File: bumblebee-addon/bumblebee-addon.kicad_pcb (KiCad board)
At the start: 2 copper layers, 19 parts, among them J1 RJ25, J2 HEADER, J3 HEADER, J4 ICSP, J5 FTDI_FLASH, J6 INTERFACE, SW1 SW_DIP_x04, U1 ATmega328P-AU, U2 MCP4902, U3 MCP4902

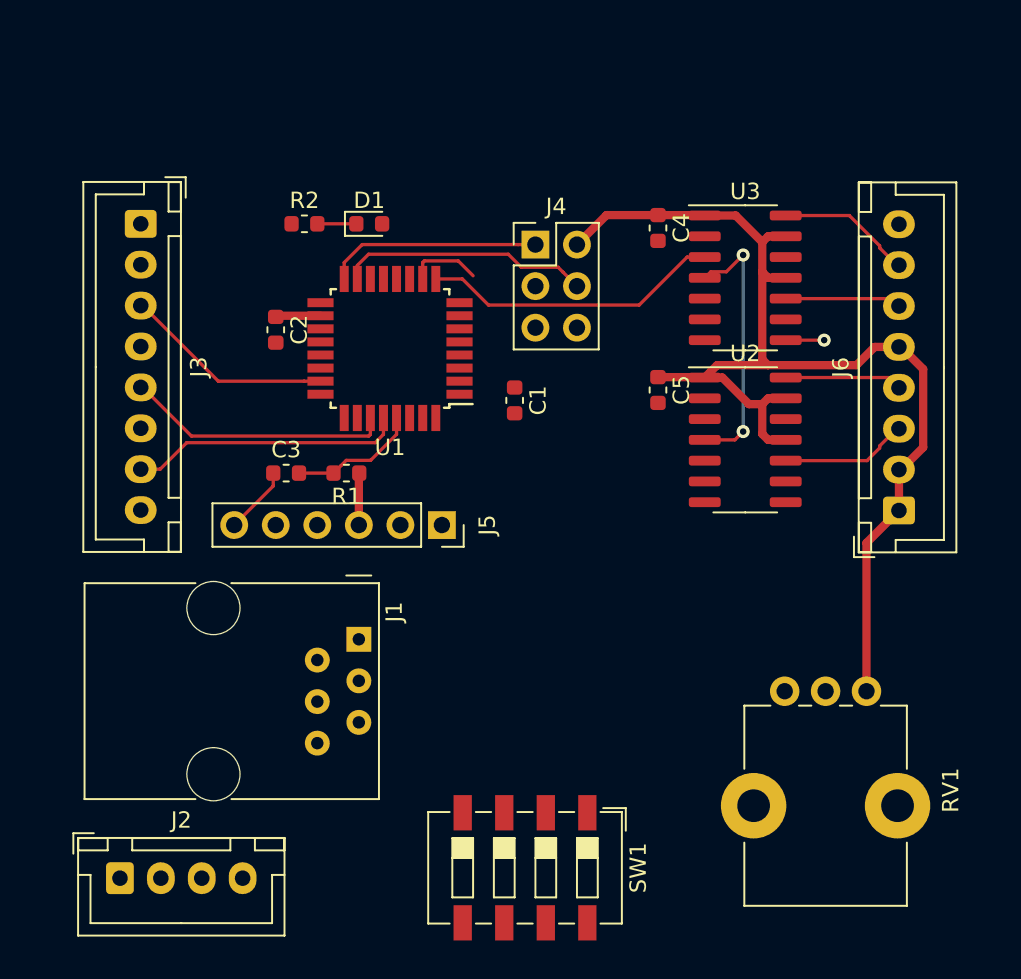
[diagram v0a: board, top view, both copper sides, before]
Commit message: Shipped new revs of all boards.
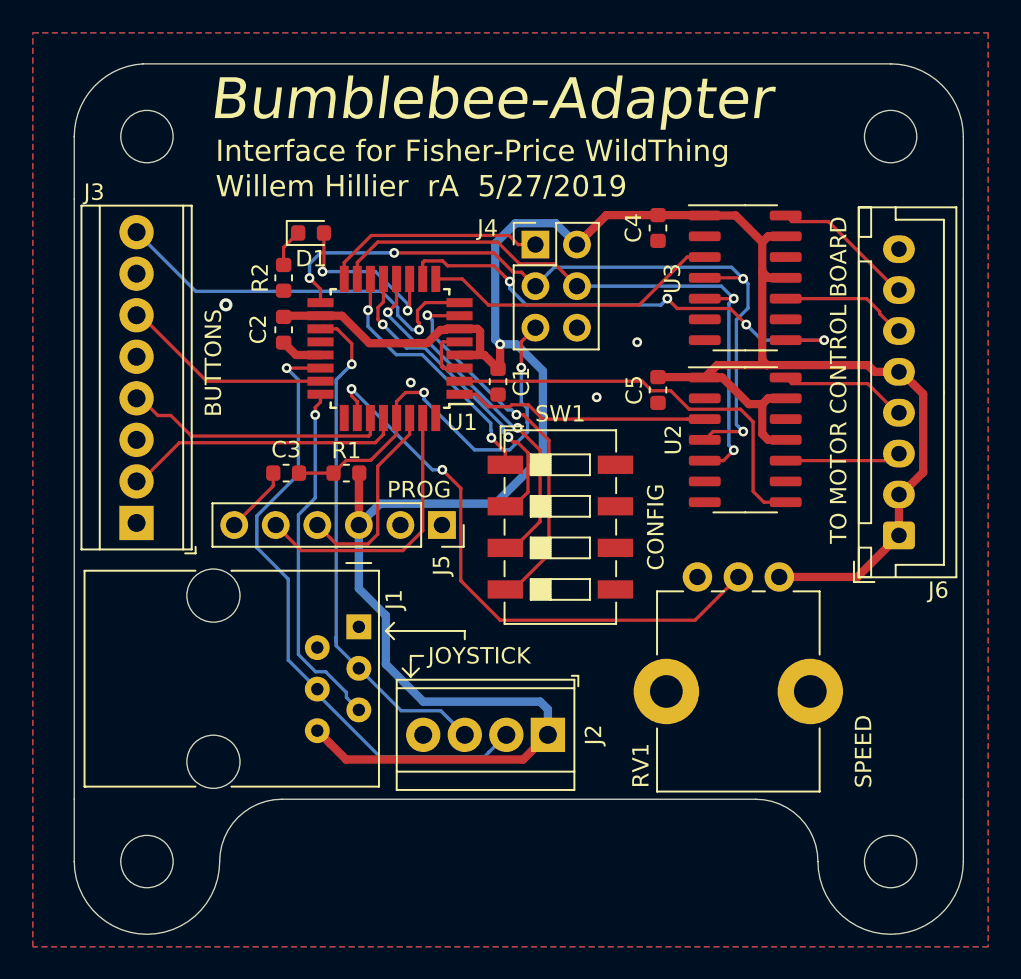
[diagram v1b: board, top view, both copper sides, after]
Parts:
- added G***: LOGO, logo:bumblebee_logo, B.Cu at (149.1, 34.8)
- added REF**: MountingHole_3.2mm_M3, MountingHole:MountingHole_3.2mm_M3, B.Cu at (127.4, 66.9)
- added REF**: MountingHole_3.2mm_M3, MountingHole:MountingHole_3.2mm_M3, F.Cu at (172.8, 66.9)
- added REF**: MountingHole_3.2mm_M3, MountingHole:MountingHole_3.2mm_M3, B.Cu at (172.8, 22.6)
- added REF**: MountingHole_3.2mm_M3, MountingHole:MountingHole_3.2mm_M3, F.Cu at (127.4, 22.6)
- J1: footprint Connector_RJ:RJ12_Amphenol_54601 -> footprints:RJ12_Amphenol_54601
- J2: footprint Connector_JST:JST_XH_B4B-XH-A_1x04_P2.50mm_Vertical -> footprints:TerminalBlock_TE_282834-4_1x04_P2.54mm_Horizontal
- J3: footprint Connector_JST:JST_XH_B8B-XH-A_1x08_P2.50mm_Vertical -> footprints:TerminalBlock_TE_282834-8_1x08_P2.54mm_Horizontal
- RV1: footprint Potentiometer_THT:Potentiometer_Bourns_PTV09A-1_Single_Vertical -> footprints:Potentiometer_Bourns_PTV09A-1_Single_Vertical
- moved J2 27.6 mm to (151.9, 59.2), turned to 180 degrees
- moved SW1 20.9 mm to (152.7, 46.5), turned to 0 degrees
- moved J3 18.3 mm to (126.7, 46.2), turned to 90 degrees
- moved RV1 8.79 mm to (161.0, 49.5)
- moved D1 3.60 mm to (137.4, 28.5)
- moved R2 3.54 mm to (135.7, 31.2), turned to 90 degrees
- moved C1 1.53 mm to (148.8, 37.6)
- moved J6 1.52 mm to (173.4, 47.0)
- moved J1 0.76 mm to (140.3, 52.6)
- moved C2 0.48 mm to (135.7, 34.4)
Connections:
- J3 pad 1: /BTN_UP -> GND
- J3 pad 2: GND -> /BTN_R
- J3 pad 3: /BTN_DN -> GND
- J3 pad 4: GND -> /BTN_L
- J3 pad 5: /BTN_L -> GND
- J3 pad 6: GND -> /BTN_DN
- J3 pad 7: /BTN_R -> GND
- J3 pad 8: GND -> /BTN_UP
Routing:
- net +3V3: track 77.5 -> 162.0 mm, vias 0 -> 1
- net /JS_X: track 0.00 -> 38.6 mm, vias 0 -> 1
- net Net-(RV1-Pad2): track 0.00 -> 35.8 mm, vias 0 -> 2
- net /JS_Y: track 0.00 -> 31.6 mm, vias 0 -> 1
- net /SCK: track 16.3 -> 45.9 mm, vias 2 -> 4
- net /DAC1_LDAC: track 0.00 -> 25.5 mm
- net /BTN_UP: track 0.00 -> 24.0 mm, vias 0 -> 1
- net /MOSI: track 15.3 -> 39.3 mm, vias 0 -> 2
- net /DAC2_LDAC: track 6.85 -> 30.5 mm, vias 1 -> 4
- net Net-(SW1-Pad4): track 0.00 -> 23.6 mm, vias 0 -> 2
- net Net-(SW1-Pad3): track 0.00 -> 22.3 mm, vias 0 -> 2
- net /JS_DETECT: track 0.00 -> 21.7 mm, vias 0 -> 1
- net Net-(SW1-Pad2): track 0.00 -> 19.5 mm, vias 0 -> 2
- net /RESET: track 7.95 -> 26.2 mm, vias 0 -> 2
- net /FTDI_RX: track 0.00 -> 17.0 mm
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- added copper zone on B.Cu, net GND
- added copper zone on F.Cu, net GND
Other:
- board outline added: 54.4 x 53.2 mm
- board text added: "3.3V JS_X JS_Y GND"
- board text added: "BUTTONS"
- board text added: "Bumblebee-Adapter"
- board text added: "CONFIG"
- board text added: "GND R-GREEN R-BLACK 3.3V L-GREEN L-BLACK 3.3V 3.3V"
- board text added: "Interface for Fisher-Price WildThing"
- board text added: "JOYSTICK"
- board text added: "PROG"
- board text added: "R L REV FOR"
- board text added: "SPEED"
- board text added: "TO MOTOR CONTROL BOARD"
- board text added: "This board is open source. For more information, hardware files, and code examples, see: https://github.com/willemcvu/Bumblebee- dual-motor-driver/tree/master/bumblebee-addon"
- board text added: "Willem Hillier rA 5/27/2019"
